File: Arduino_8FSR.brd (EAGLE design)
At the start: 74.9 x 64.4 mm, 17 parts, among them IC1 7805TV, IC2 UA741P, U1 HCF4051BEY, X2 TSW-117-08-G-S, X3 TSW-117-08-G-S, X4 057-006-1, X5 057-010-1

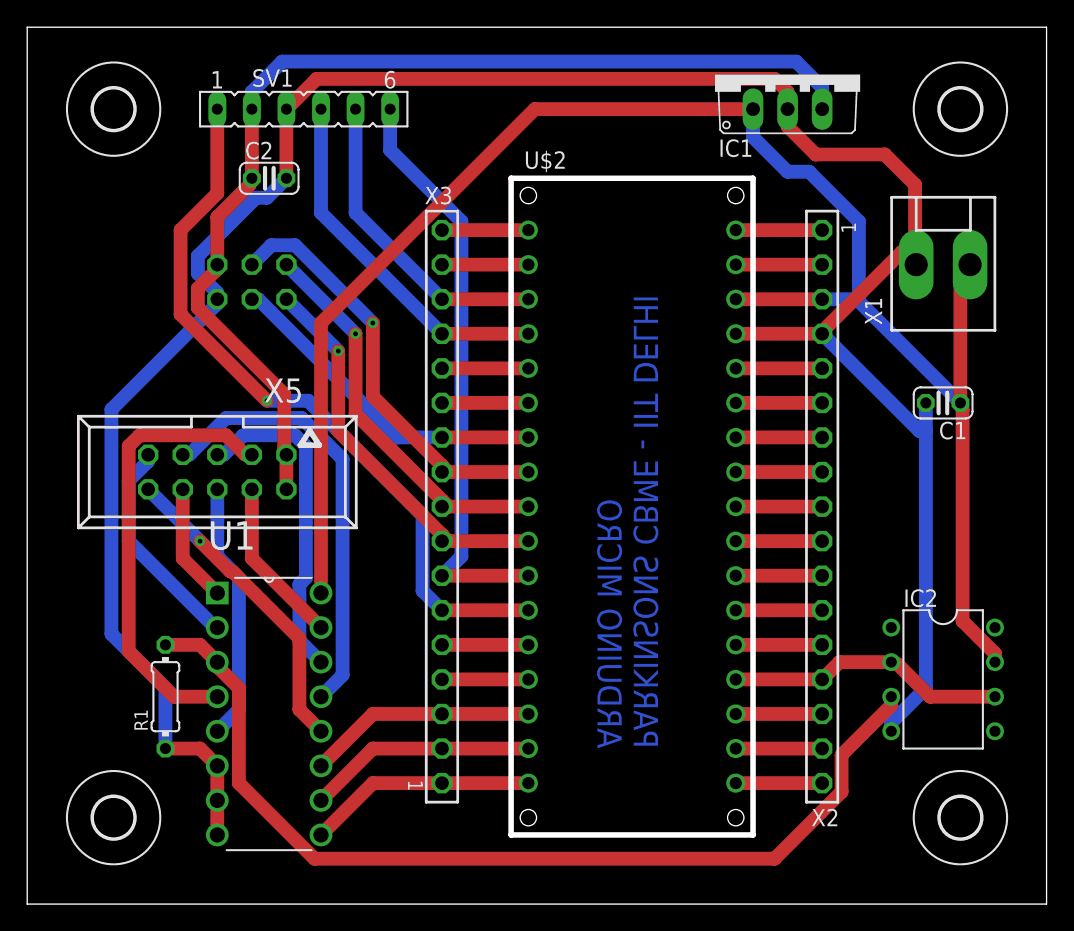
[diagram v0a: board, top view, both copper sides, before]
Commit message: Final Version
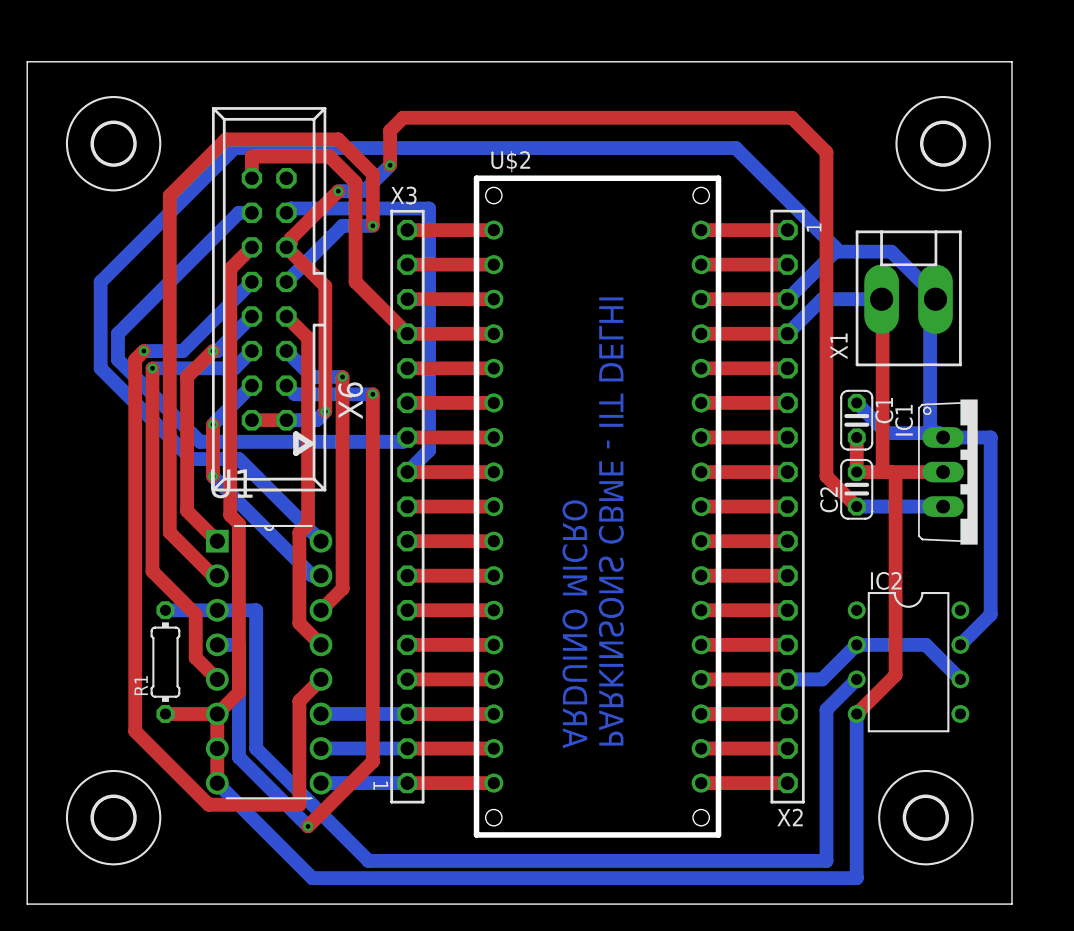
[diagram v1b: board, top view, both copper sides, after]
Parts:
- removed SV1: (no value), con-lsta:FE06
- removed X4: 057-006-1, con-panduit:057-006-1
- removed X5: 057-010-1, con-panduit:057-010-1
- added X6: 057-016-1, con-panduit:057-016-1
- moved C2 48.9 mm to (61.0, 30.5), turned to 90 degrees
- moved IC1 32.4 mm to (69.8, 31.8), turned to 270 degrees
- moved C1 6.48 mm to (61.0, 35.6), turned to 270 degrees
- moved U1 3.81 mm to (21.6, 8.89)
- moved X1 3.59 mm to (64.8, 44.5)
- moved IC2 2.84 mm to (64.8, 17.8)
- moved H3 2.84 mm to (67.3, 55.9)
- moved R1 2.54 mm to (10.2, 17.8)
- moved H2 2.54 mm to (6.35, 55.9)
- moved U$2 2.54 mm to (33.0, 7.62)
- moved X2 2.54 mm to (55.9, 29.2)
- moved X3 2.54 mm to (27.9, 29.2)
- moved H4 2.54 mm to (66.0, 6.35)
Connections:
- removed net AD0: U$2.D4, X3.9, X4.5
- removed net EN: SV1.1, U$2.D7, X3.6
- removed net RXTX: SV1.5, U$2.TX, X3.15
- removed net STATE: SV1.6, U$2.D6, X3.7
- removed net TXRX: SV1.4, U$2.RX, X3.14
- new net N$10: U$2.TX, X3.15
- new net N$4: U$2.D5, X3.8
- new net N$7: U$2.D6, X3.7
- new net N$8: U$2.D7, X3.6
- new net N$9: U$2.D4, X3.9
- new net NC: X6.15
- net GND: now also X6.12; no longer SV1.3, X4.2
- net INT: now also U$2.RX, X3.14, X6.16; no longer U$2.D5, X3.8, X4.6
- net IP1: now also X6.3; no longer X5.3
- net IP2: now also X6.4; no longer X5.4
- net IP3: now also X6.5; no longer X5.5
- net IP4: now also X6.6; no longer X5.6
- net IP5: now also X6.7; no longer X5.7
- net IP6: now also X6.8; no longer X5.8
- net IP7: now also X6.9; no longer X5.9
- net IP8: now also X6.10; no longer X5.10
- net SCL: now also X6.13; no longer X4.3
- net SDA: now also X6.14; no longer X4.4
- net VCC_5V: now also X6.1, X6.11, X6.2; no longer SV1.2, X4.1, X5.1, X5.2
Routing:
- net EN: track 54.0 -> 0.00 mm, vias 1 -> 0
- net STATE: track 43.4 -> 0.00 mm
- net IP7: track 16.1 -> 59.1 mm, vias 0 -> 1
- net IP8: track 23.1 -> 62.4 mm
- net AD0: track 29.1 -> 0.00 mm, vias 1 -> 0
- net TXRX: track 26.5 -> 0.00 mm
- net IP1: track 32.9 -> 57.4 mm, vias 0 -> 2
- net RXTX: track 23.0 -> 0.00 mm
- net SDA: track 24.5 -> 45.7 mm
- net VCC: track 126.6 -> 147.7 mm
- net VCC_5V: track 78.6 -> 98.6 mm, vias 0 -> 3
- net IP4: track 19.1 -> 32.7 mm, vias 0 -> 1
- net GND: track 174.7 -> 161.8 mm
- net IP6: track 8.67 -> 19.6 mm, vias 0 -> 1
- net IP2: track 12.3 -> 18.8 mm, vias 0 -> 2
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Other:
- board size 74.9 x 64.4 mm -> 72.4 x 61.9 mm
